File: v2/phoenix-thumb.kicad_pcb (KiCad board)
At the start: 2 copper layers, 39.9 x 27.1 mm, 5 parts

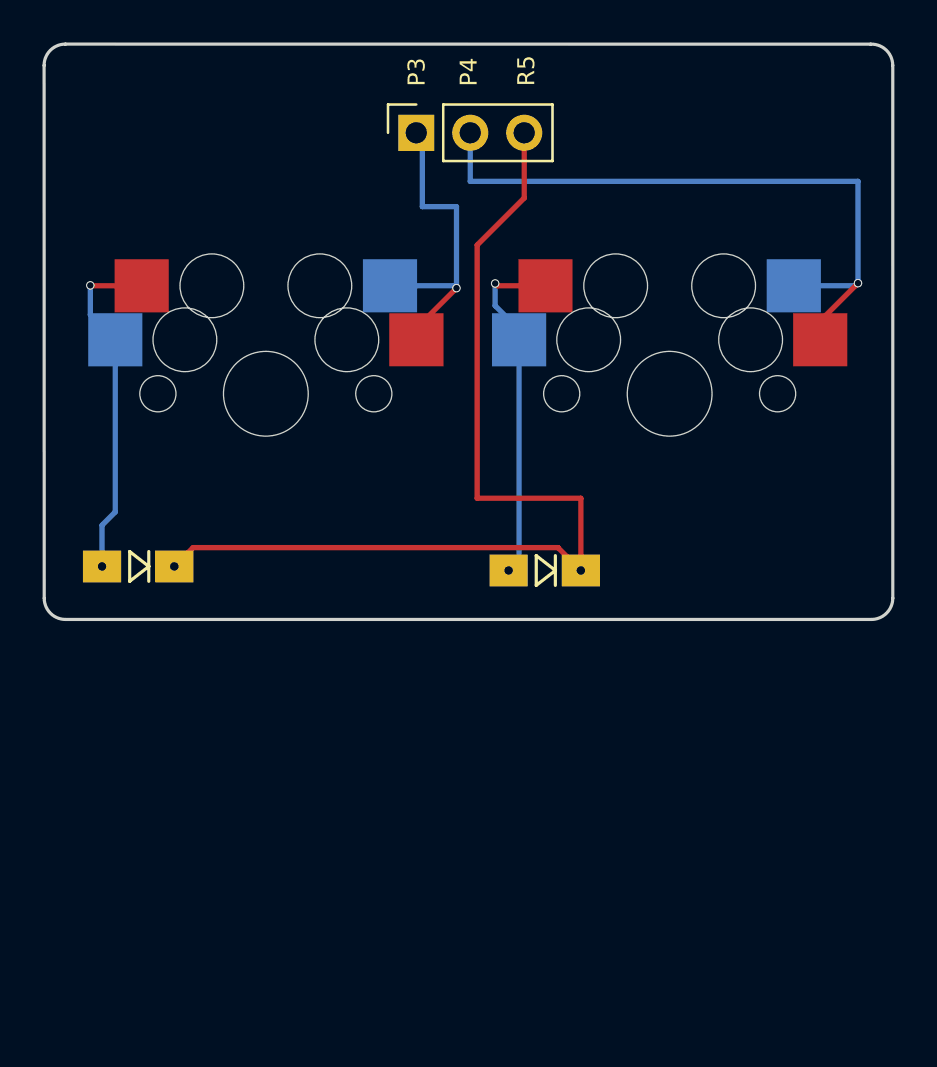
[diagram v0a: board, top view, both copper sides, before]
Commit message: thumb
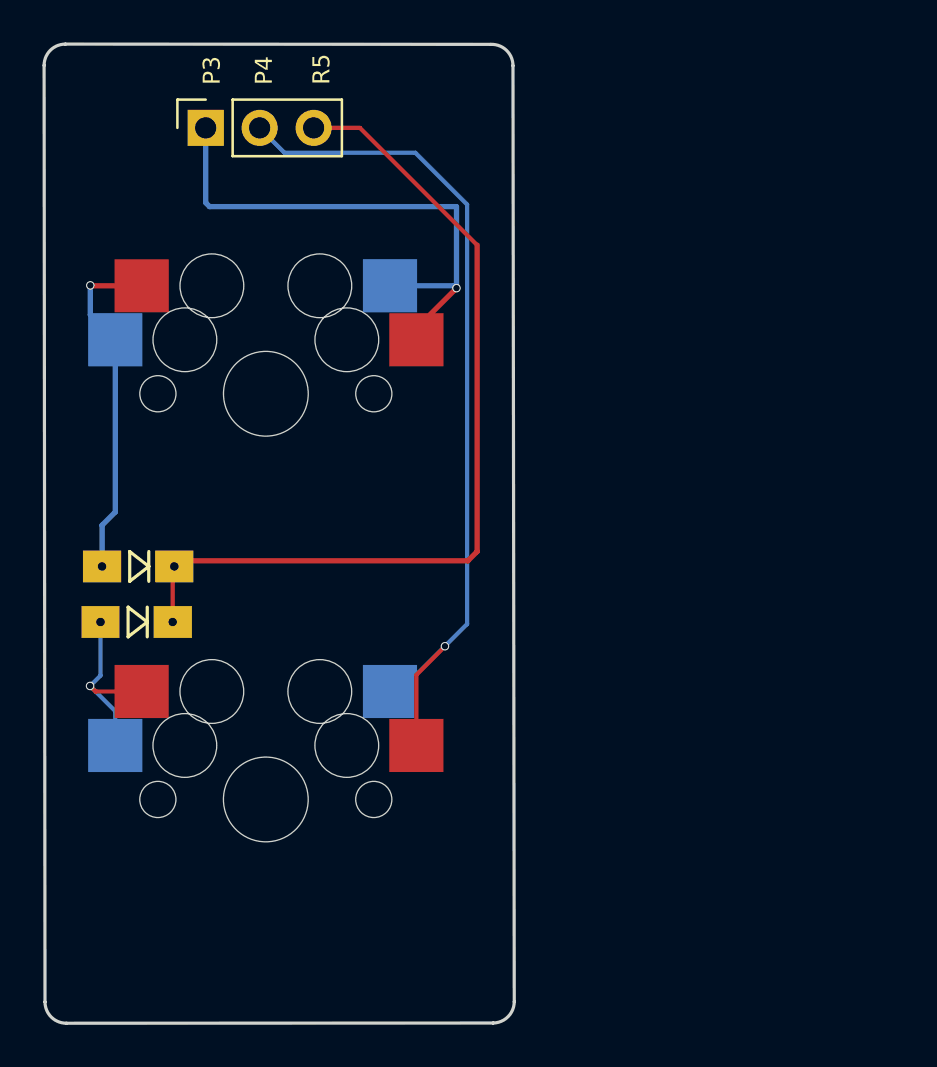
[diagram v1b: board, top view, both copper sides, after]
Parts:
- moved S7 26.9 mm to (140.4, 161.5)
- moved D25 19.4 mm to (134.3, 153.2)
- moved REF** 9.91 mm to (137.6, 129.9)
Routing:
- net P3: track 15.4 -> 25.6 mm
- net P4: track 31.8 -> 41.2 mm
- net R31: track 16.6 -> 9.04 mm
- net row5: track 46.8 -> 41.9 mm
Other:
- board size 39.9 x 27.1 mm -> 22.1 x 46.1 mm
